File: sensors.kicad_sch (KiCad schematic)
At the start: 8 parts, among them U3 LSM6DSOX, U4 LIS2MDL

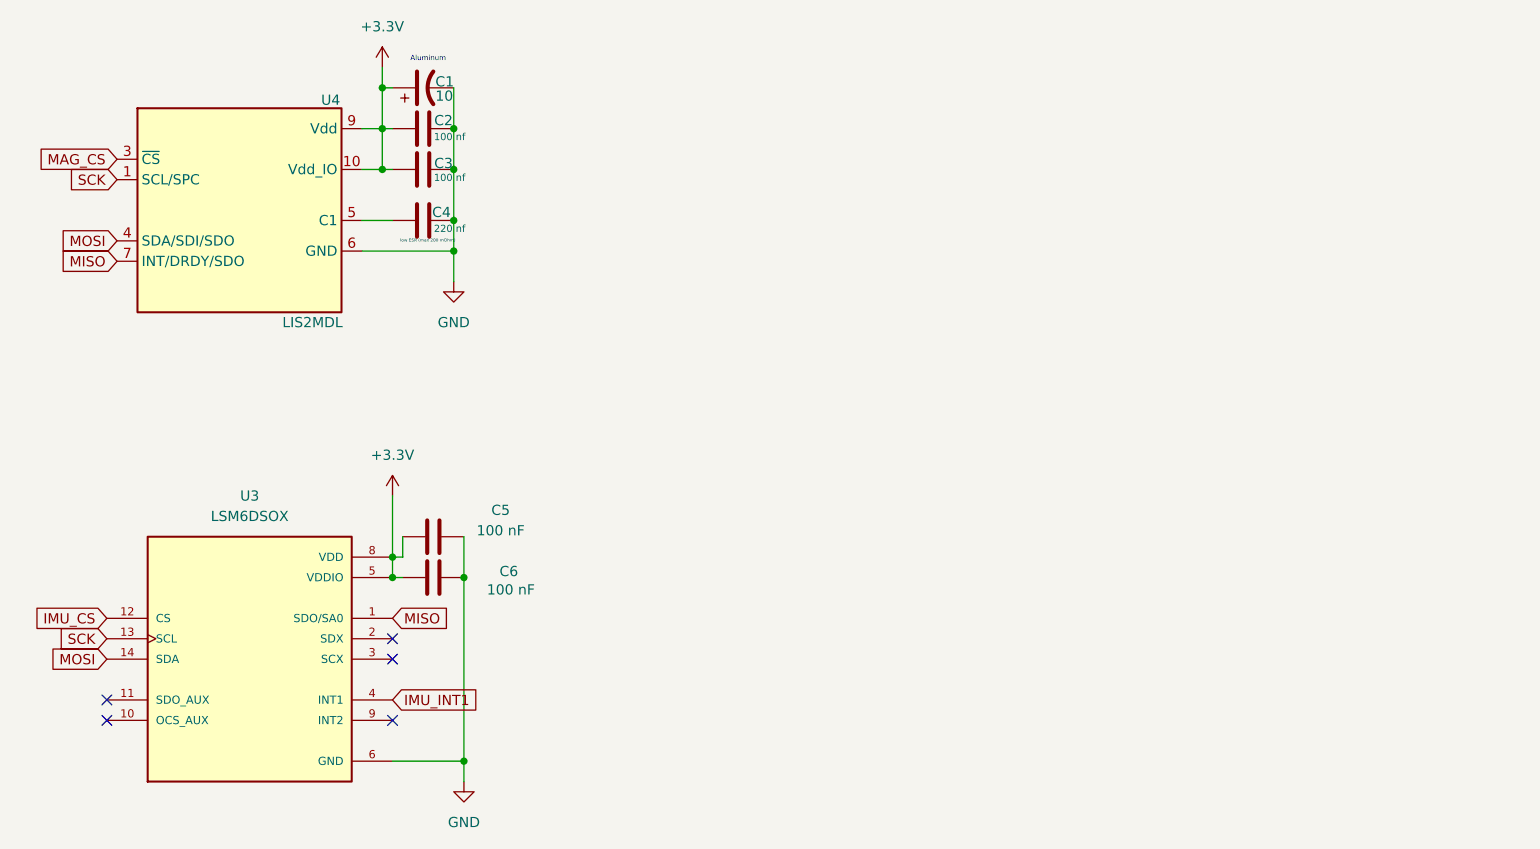
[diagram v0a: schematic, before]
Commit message: Add files via upload
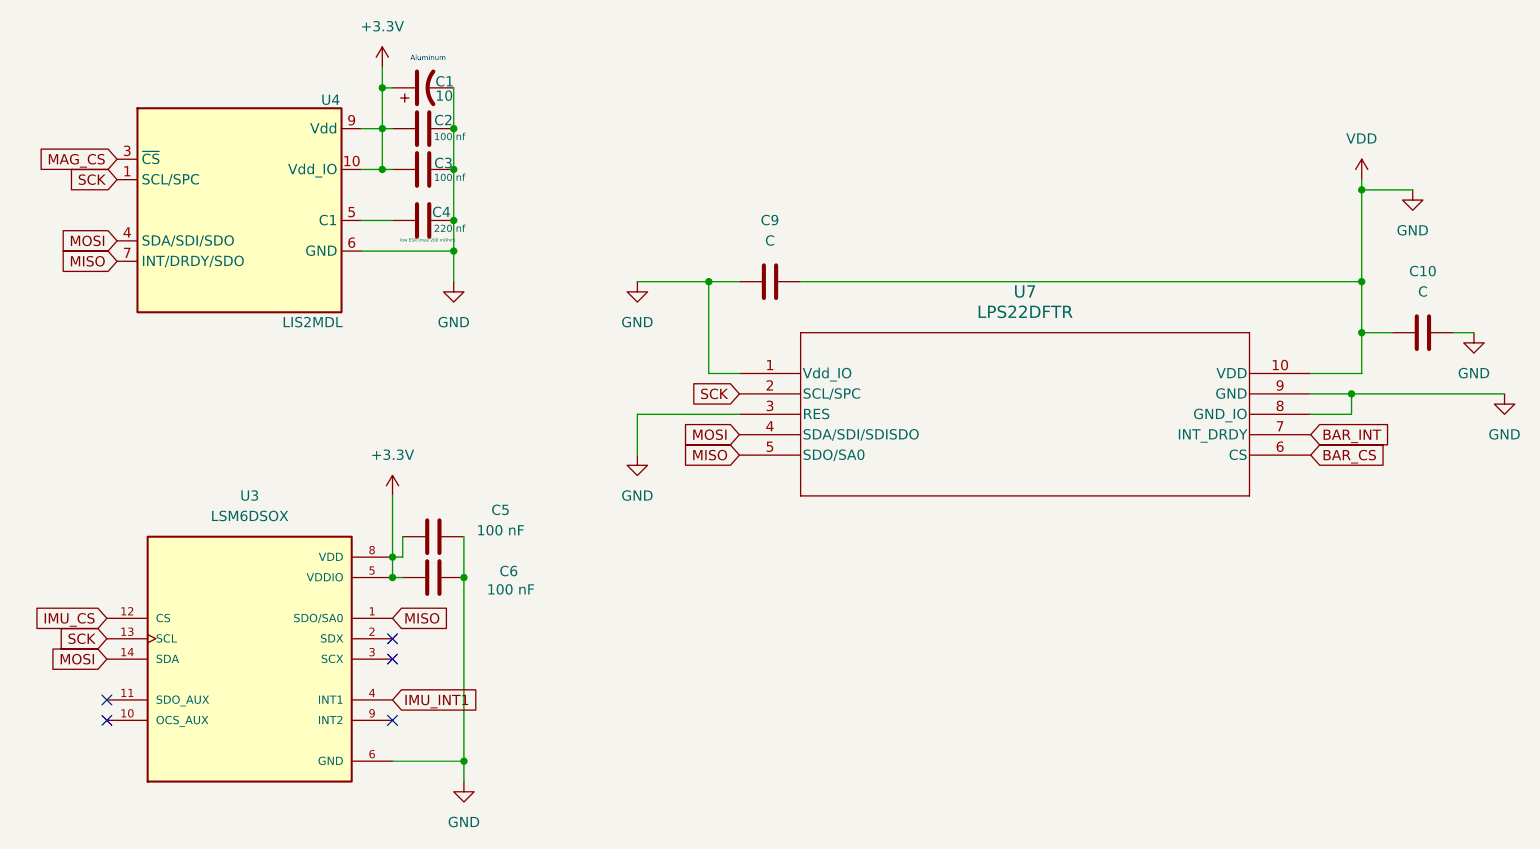
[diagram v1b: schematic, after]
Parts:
- added C10, C9: C, Capacitor_SMD:C_0201_0603Metric, symbol Device:C
- added U7: LPS22DFTR, QFN_22DFTR_STM, symbol New_Library:LPS22DFTR
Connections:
- net GND: now also C10.1, C10.2, C9.1, C9.2, U7.1 (Vdd_IO), U7.10 (VDD), U7.3 (RES), U7.8 (GND_IO), U7.9 (GND)
- net MISO: now also U7.5 (SDO/SA0)
- net MOSI: now also U7.4 (SDA/SDI/SDISDO)
- net SCK: now also U7.2 (SCL/SPC)
- new net BAR_CS: U7.6 (CS)
- new net BAR_INT: U7.7 (INT_DRDY)
